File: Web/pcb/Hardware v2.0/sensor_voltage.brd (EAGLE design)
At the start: 74.9 x 32.7 mm, 18 parts, among them IC1 OPA344, J1 22-27-2041-04

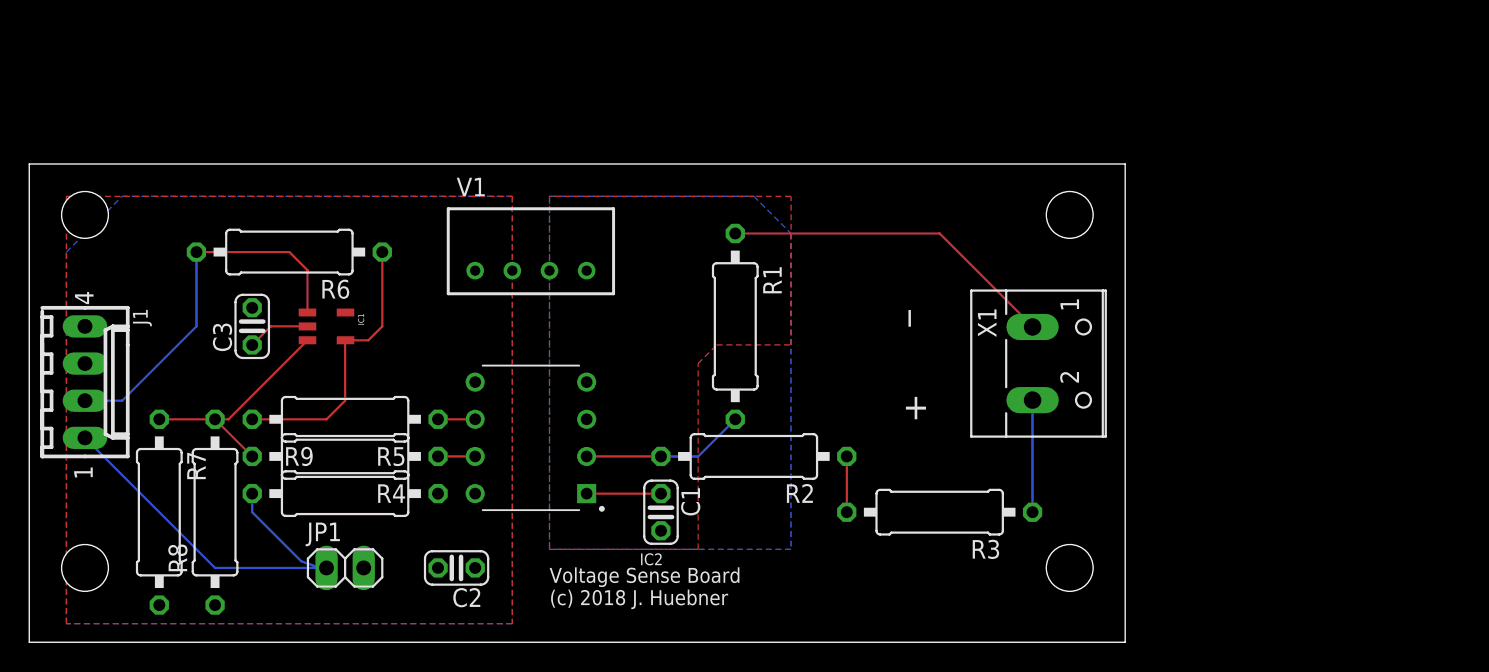
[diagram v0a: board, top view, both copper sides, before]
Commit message: updates
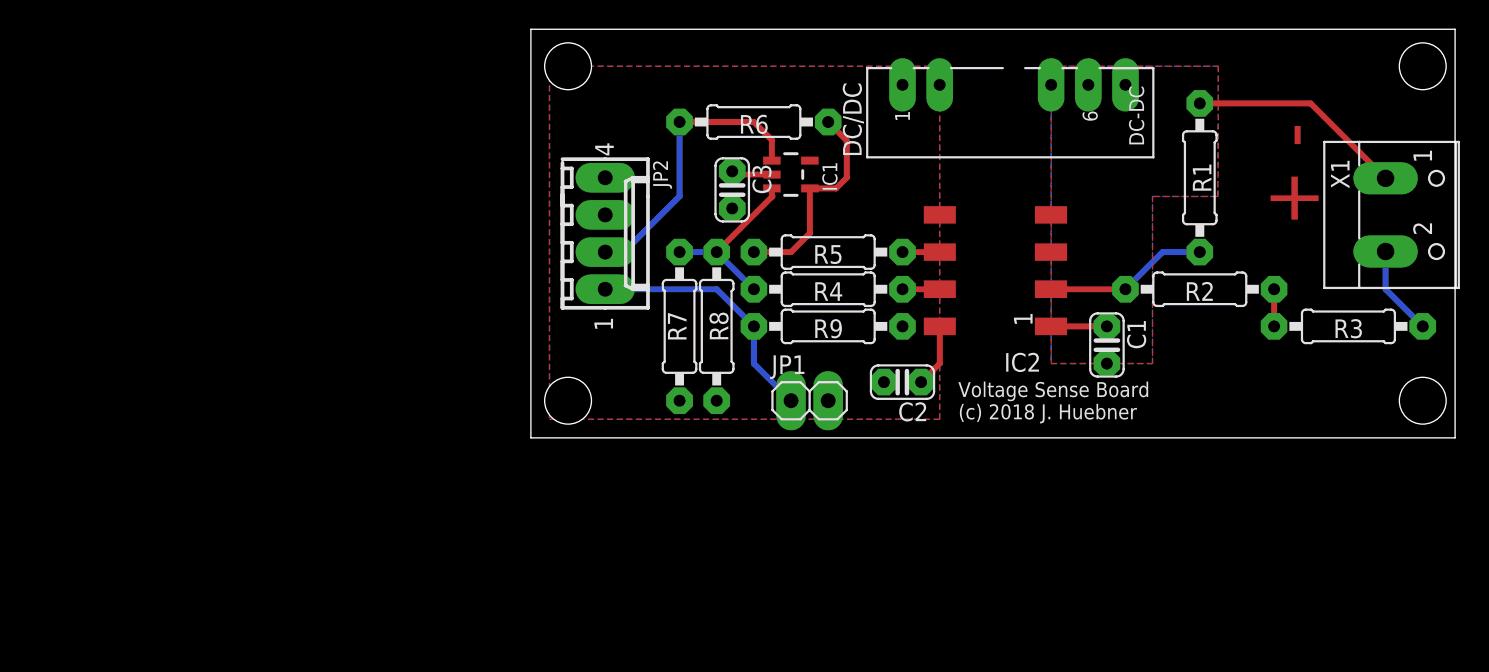
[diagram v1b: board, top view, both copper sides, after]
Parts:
- removed J1: 22-27-2041-04, con-molex:6410-04
- removed V1: TME0505S, traco-electronic:TME
- added DC/DC: (no value), dc-dc-converter:NMA
- added JP2: 22-27-2041-04, con-molex:6410-04
- C1, C2, C3: value 1uF -> 1µ
- IC1: device OPA344:SOT23-5 -> SparkFun-AnalogIC:SOT23-5
- IC2: value (none) -> SI8920; device SI8920BC:SI8920BC -> silabs:DIP8
- R1: value 470 -> 500; device rcl:0309/12 -> rcl:0207/10
- R2, R3, R4, R5, R6, R7, R8, R9: device rcl:0309/12 -> rcl:0207/10
- moved R7 37.8 mm to (10.2, 7.62), turned to 90 degrees
- moved R8 36.6 mm to (12.7, 7.62), turned to 270 degrees
- moved R4 34.9 mm to (20.3, 10.2)
- moved R5 34.9 mm to (20.3, 12.7)
- moved R9 34.9 mm to (20.3, 7.62), turned to 180 degrees
- moved C3 34.1 mm to (13.8, 16.9), turned to 270 degrees
- moved IC2 33.7 mm to (31.8, 11.4), turned to 90 degrees
- moved JP1 33.7 mm to (19.1, 2.54)
- moved IC1 33.4 mm to (17.8, 18.0)
- moved R1 33.3 mm to (45.7, 17.8)
- moved C2 33.0 mm to (25.4, 3.81)
- moved R6 33.0 mm to (15.2, 21.6)
- moved C1 32.6 mm to (39.4, 6.35)
- moved R2 32.6 mm to (45.7, 10.2)
- moved R3 30.7 mm to (55.9, 7.62)
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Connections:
- removed net N$3 (its old number): IC1.1, J1.2, R6.2
- removed net N$4 (its old number): IC1.3, R4.2, R7.1, R8.2
- removed net N$5 (its old number): J1.1, JP1.1, R9.1
- new net N$6: IC1.1, JP2.2, R6.2
- new net N$8: IC1.3, R4.2, R7.2, R8.1
- new net N$9: JP1.1, JP2.1, R9.2
- net GND: now also DC/DC.2, JP1.2, JP2.3, R8.2; no longer J1.3, R8.1, R9.2, V1.1
- net GND1: now also DC/DC.4; no longer V1.3
- net VCC: now also DC/DC.1, JP2.4, R7.1, R9.1; no longer J1.4, JP1.2, R7.2, V1.2
- net VCCIO: now also DC/DC.6; no longer V1.4
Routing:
- net N$5 (its old number): track 28.0 -> 0.00 mm
- net N$3 (its old number): track 25.8 -> 0.00 mm
- net N$6: track 0.00 -> 20.0 mm
- net N$9: track 0.00 -> 17.3 mm
- net N$4 (its old number): track 16.0 -> 0.00 mm
- net N$8: track 0.00 -> 12.1 mm
- net GND1: track 23.0 -> 14.8 mm
- net N$7: track 19.0 -> 14.6 mm
- net VCC: track 4.31 -> 7.14 mm
- net N$3: track 7.66 -> 6.17 mm
- net N$2: track 3.81 -> 2.54 mm
- net VCCIO: track 5.08 -> 3.82 mm
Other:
- board size 74.9 x 32.7 mm -> 63.2 x 27.9 mm
- board text added: "+ -"
- board text removed: "+"
- board text removed: "_"
